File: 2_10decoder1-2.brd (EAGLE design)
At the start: 26.6 x 29.4 mm, 15 parts, among them T1 BC847, T2 BC847

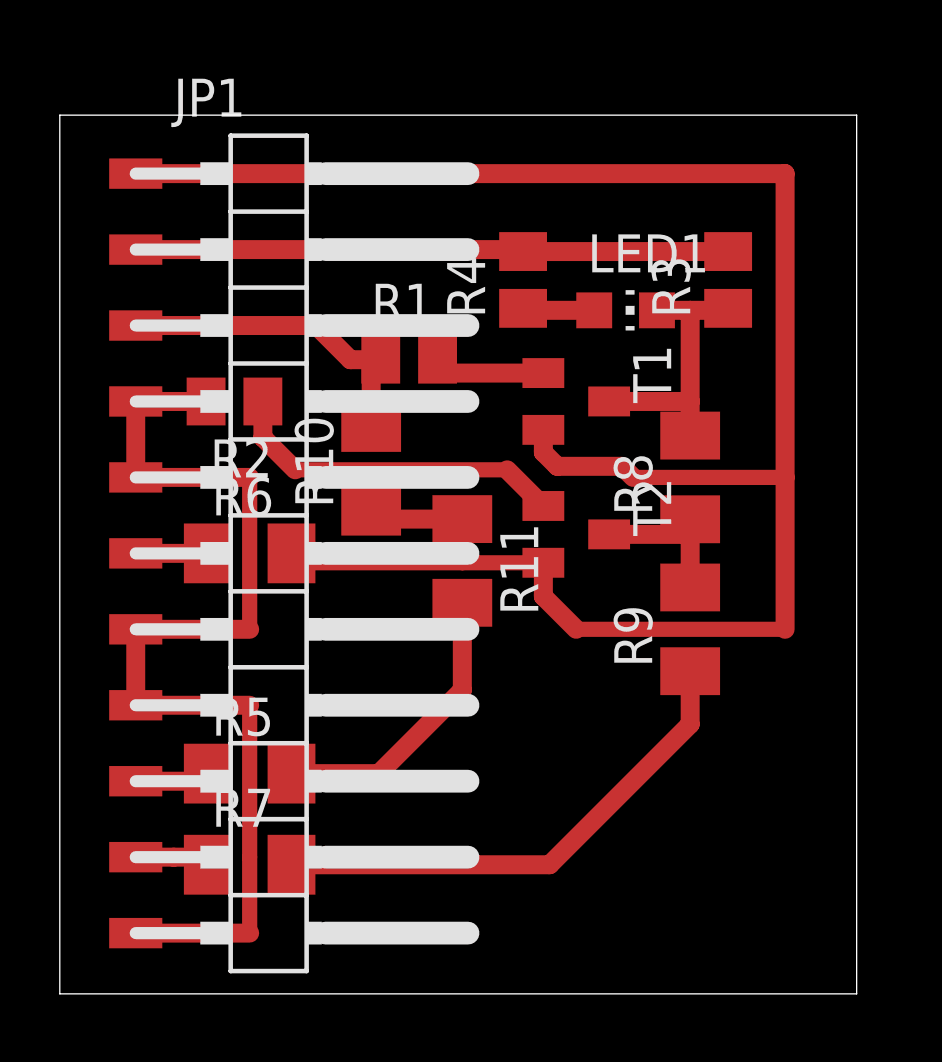
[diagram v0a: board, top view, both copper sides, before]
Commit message: general fix 1-2 decoder
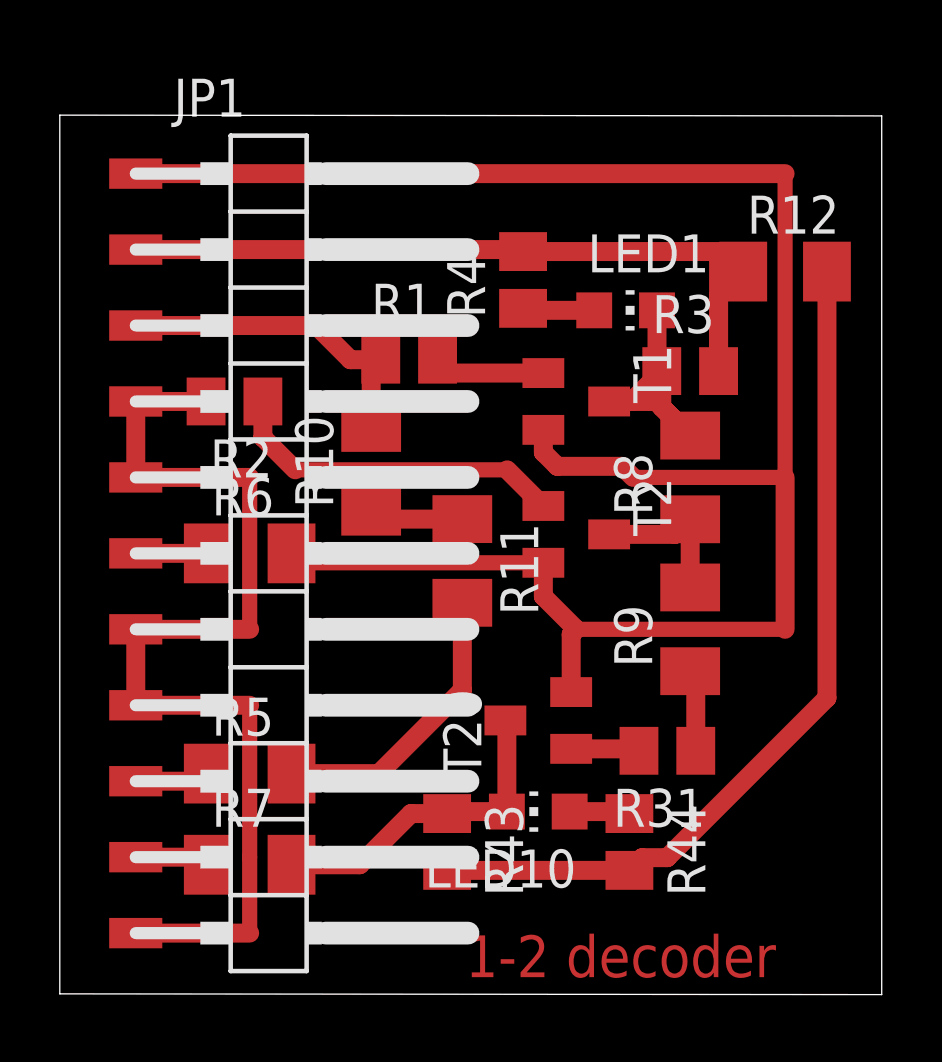
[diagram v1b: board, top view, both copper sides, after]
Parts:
- added LED10: (no value), led:CHIP-LED0805
- added R12: 0R, rcl:M1206
- added R31: 10k, resistor:M0805
- added R43: 3K9, resistor:M0805
- added R44: (no value), resistor:M0805
- added T20: BC847, transistor-neu-to92:SOT23
- moved R3 3.30 mm to (21.1, 64.5), turned to 0 degrees
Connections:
- new net N$35: R31.2, T20.1
- new net N$49: LED10.A, R44.1
- new net N$50: LED1.C, R3.1, R31.1, R8.1, R8.2, R9.1, R9.2, T1.3, T2.3
- net B: now also LED10.C, R43.1, T20.3; no longer LED1.C, R3.1, R8.1, R8.2, R9.1, R9.2, T1.3, T2.3
- net GND: now also T20.2
- net VCC: now also R12.1, R12.2, R43.2, R44.2
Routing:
- net VCC: track 19.8 -> 57.7 mm
- net B: track 34.7 -> 13.5 mm
- net N$50: track 0.00 -> 18.5 mm
- net N$35: track 0.00 -> 2.30 mm
- net GND: track 66.9 -> 69.1 mm
- net N$49: track 0.00 -> 2.03 mm
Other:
- board size 26.6 x 29.4 mm -> 27.5 x 29.4 mm
- board text added: "1-2 decoder"
